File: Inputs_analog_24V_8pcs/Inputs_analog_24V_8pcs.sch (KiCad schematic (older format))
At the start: 14 parts, among them J1 Screw_Terminal_01x02, J2 Screw_Terminal_01x02, J3 Screw_Terminal_01x06, U1 SN74HC14N, U2 SN74HC14N, U3 74HC151N.652

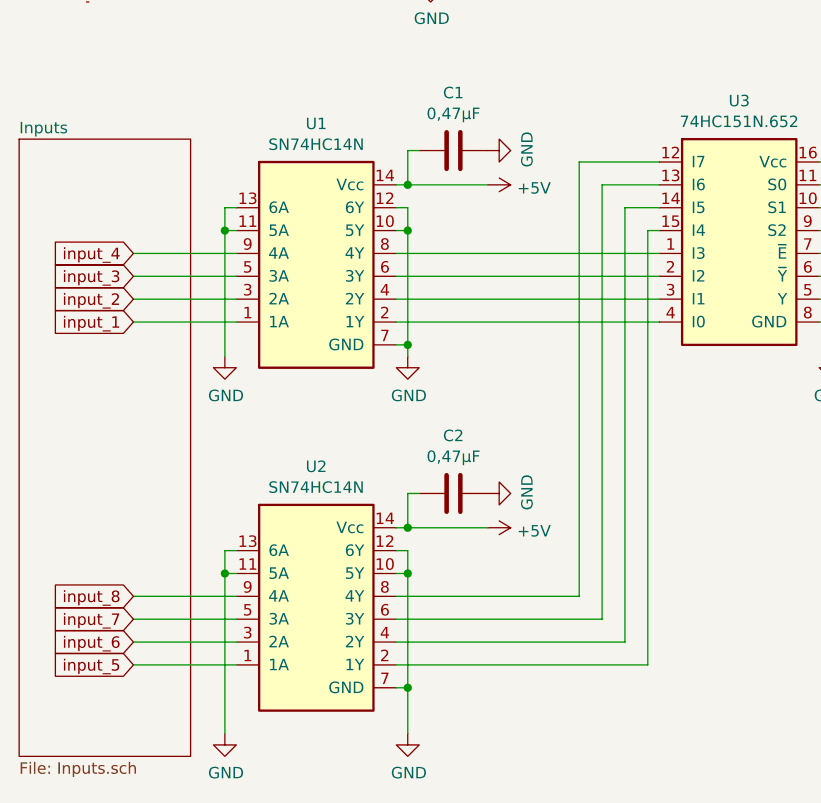
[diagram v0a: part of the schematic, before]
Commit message: Update pcb
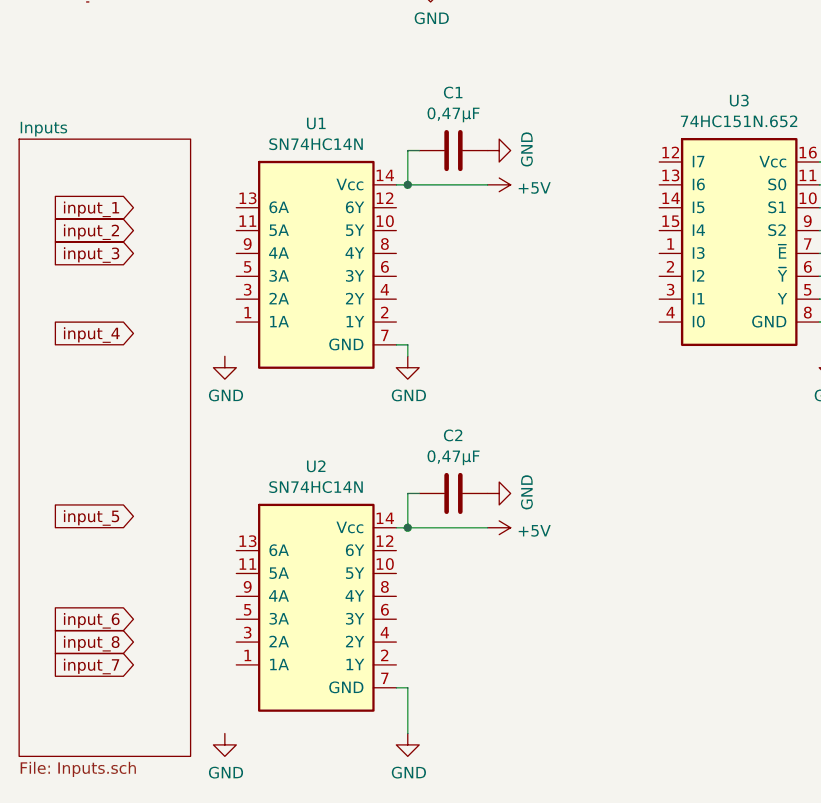
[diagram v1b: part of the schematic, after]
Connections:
- net GND: no longer U1.10 (5Y), U1.11 (5A), U1.12 (6Y), U1.13 (6A), U2.10 (5Y), U2.11 (5A), U2.12 (6Y), U2.13 (6A)
- net input_1: no longer U1.1 (1A)
- net input_2: no longer U1.3 (2A)
- net input_3: no longer U1.5 (3A)
- net input_4: no longer U1.9 (4A)
- net input_5: no longer U2.1 (1A)
- net input_6: no longer U2.3 (2A)
- net input_7: no longer U2.5 (3A)
- net input_8: no longer U2.9 (4A)
- net at U1.2 (1Y): no longer U3.4 (I0)
- net at U1.4 (2Y): no longer U3.3 (I1)
- net at U1.6 (3Y): no longer U3.2 (I2)
- net at U1.8 (4Y): no longer U3.1 (I3)
- net at U2.2 (1Y): no longer U3.15 (I4)
- net at U2.4 (2Y): no longer U3.14 (I5)
- net at U2.6 (3Y): no longer U3.13 (I6)
- net at U2.8 (4Y): no longer U3.12 (I7)
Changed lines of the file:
@@
 F1 "Inputs.sch" 50
 $EndSheet
-Text GLabel 1500 3900 0    50   Input ~ 0
+Text GLabel 1500 3400 0    50   Input ~ 0
 input_1
-Text GLabel 1500 3800 0    50   Input ~ 0
+Text GLabel 1500 3500 0    50   Input ~ 0
 input_2
-Text GLabel 1500 3700 0    50   Input ~ 0
+Text GLabel 1500 3600 0    50   Input ~ 0
 input_3
-Text GLabel 1500 3600 0    50   Input ~ 0
+Text GLabel 1500 3950 0    50   Input ~ 0
 input_4
+Text GLabel 1500 4750 0    50   Input ~ 0
+input_5
+Text GLabel 1500 5200 0    50   Input ~ 0
+input_6
 Text GLabel 1500 5400 0    50   Input ~ 0
-input_5
+input_7
 Text GLabel 1500 5300 0    50   Input ~ 0
-input_6
-Wire Wire Line
-	1500 3600 1950 3600
-Wire Wire Line
-	1500 3700 1950 3700
-Wire Wire Line
-	1500 3800 1950 3800
-Wire Wire Line
-	1500 3900 1950 3900
-Text GLabel 1500 5200 0    50   Input ~ 0
-input_7
-Text GLabel 1500 5100 0    50   Input ~ 0
 input_8
-Wire Wire Line
-	1500 5300 1950 5300
-Wire Wire Line
-	1500 5400 1950 5400
 $Comp
 L power:GND #PWR04
@@
 	1    0    0    -1
 $EndComp
-Wire Wire Line
-	1900 4900 1950 4900
-Wire Wire Line
-	1950 5000 1900 5000
-Connection ~ 1900 5000
-Wire Wire Line
-	1900 5000 1900 4900
 $Comp
 L power:+5V #PWR09
@@
 Wire Wire Line
 	2700 5500 2700 5700
-Connection ~ 2700 5500
-Wire Wire Line
-	2650 5000 2700 5000
-Wire Wire Line
-	2650 4900 2700 4900
-Wire Wire Line
-	2700 4900 2700 5000
-Connection ~ 2700 5000
 $Comp
 L power:+5V #PWR011
@@
 Wire Wire Line
 	4550 3900 4550 4050
-Wire Wire Line
-	1900 5000 1900 5700
-Wire Wire Line
-	1500 5200 1950 5200
-Wire Wire Line
-	1500 5100 1950 5100
 $Comp
 L power:GND #PWR03
@@
 $EndComp
 Wire Wire Line
-	1950 3500 1900 3500
-Wire Wire Line
-	1900 3500 1900 4050
-Wire Wire Line
-	1950 3400 1900 3400
-Wire Wire Line
-	1900 3400 1900 3500
-Connection ~ 1900 3500
-Wire Wire Line
-	2650 3500 2700 3500
-Wire Wire Line
-	2700 3500 2700 4000
-Connection ~ 2700 4000
-Wire Wire Line
-	2650 3400 2700 3400
-Wire Wire Line
-	2700 3400 2700 3500
-Connection ~ 2700 3500
-Wire Wire Line
-	3750 5400 3750 3500
-Wire Wire Line
-	3750 3500 3800 3500
-Wire Wire Line
-	3650 5300 3650 3400
-Wire Wire Line
-	3650 3400 3800 3400
-Wire Wire Line
-	3800 3300 3550 3300
-Wire Wire Line
-	3550 3300 3550 5200
-Wire Wire Line
-	3450 5100 3450 3200
-Wire Wire Line
-	3450 3200 3800 3200
-Wire Wire Line
-	2650 5100 3450 5100
-Wire Wire Line
-	2650 5200 3550 5200
-Wire Wire Line
-	2650 5300 3650 5300
-Wire Wire Line
-	2700 5000 2700 5500
-Wire Wire Line
-	3750 5400 2650 5400
-Wire Wire Line
-	2650 3600 3800 3600
-Wire Wire Line
-	2650 3700 3800 3700
-Wire Wire Line
-	2650 3800 3800 3800
-Wire Wire Line
-	2650 3900 3800 3900
-Wire Wire Line
 	4500 3300 4750 3300

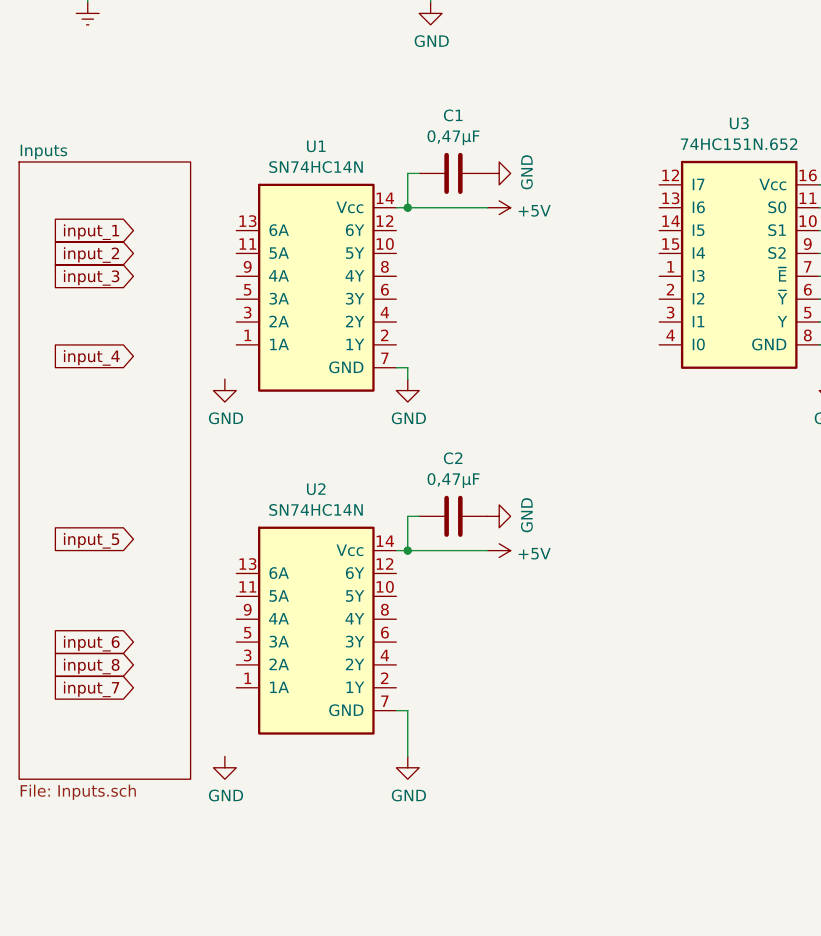
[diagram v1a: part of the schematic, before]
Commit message: Update pcb
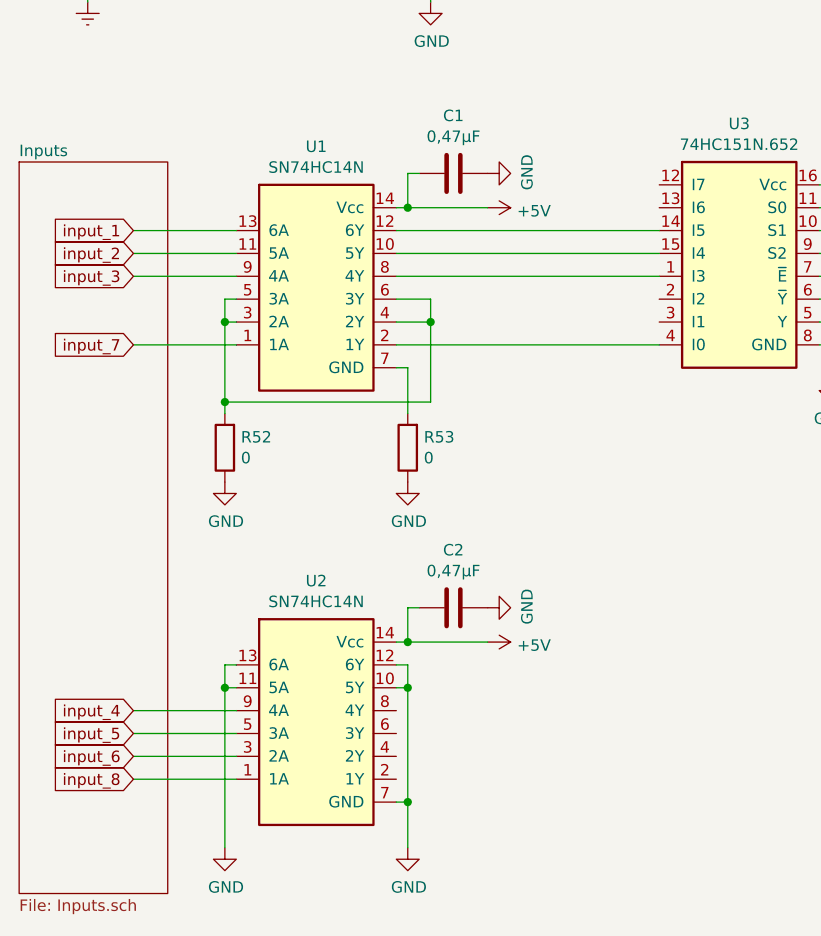
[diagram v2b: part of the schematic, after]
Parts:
- added R52, R53: 0, Resistor_THT:R_Axial_DIN0207_L6.3mm_D2.5mm_P7.62mm_Horizontal, symbol Device:R
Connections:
- net GND: now also U2.10 (5Y), U2.11 (5A), U2.12 (6Y), U2.13 (6A), R52.1, R53.1; no longer U1.7 (GND)
- net input_1: now also U1.13 (6A)
- net input_2: now also U1.11 (5A)
- net input_3: now also U1.9 (4A)
- net input_4: now also U2.9 (4A)
- net input_5: now also U2.5 (3A)
- net input_6: now also U2.3 (2A)
- net input_7: now also U1.1 (1A)
- net input_8: now also U2.1 (1A)
- net at U1.10 (5Y): now also U3.15 (I4)
- net at U1.12 (6Y): now also U3.14 (I5)
- net at U1.2 (1Y): now also U3.4 (I0)
- net at U1.3 (2A): now also U1.4 (2Y), U1.5 (3A), U1.6 (3Y), R52.2
- net at U1.8 (4Y): now also U3.1 (I3)
- new net: R53.2, U1.7 (GND)
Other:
- moved on the sheet: C2, U2
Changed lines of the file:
@@
 L Inputs_library:SN74HC14N U2
 U 1 1 5EA6DB6E
-P 2550 5950
-F 0 "U2" H 2300 7367 50  0000 C CNN
-F 1 "SN74HC14N" H 2300 7276 50  0000 C CNN
-F 2 "Package_DIP:DIP-14_W7.62mm" H 2550 5950 50  0001 C CNN
-F 3 "" H 2550 5950 50  0001 C CNN
-	1    2550 5950
+P 2550 6350
+F 0 "U2" H 2300 7767 50  0000 C CNN
+F 1 "SN74HC14N" H 2300 7676 50  0000 C CNN
+F 2 "Package_DIP:DIP-14_W7.62mm" H 2550 6350 50  0001 C CNN
+F 3 "" H 2550 6350 50  0001 C CNN
+	1    2550 6350
 	1    0    0    -1
 $EndComp
@@
 $EndComp
 $Sheet
-S 1000 3100 750  2700
+S 1000 3100 650  3200
 U 5EB670BF
 F0 "Inputs" 50
@@
 Text GLabel 1500 3600 0    50   Input ~ 0
 input_3
-Text GLabel 1500 3950 0    50   Input ~ 0
+Text GLabel 1500 5500 0    50   Input ~ 0
 input_4
-Text GLabel 1500 4750 0    50   Input ~ 0
+Text GLabel 1500 5600 0    50   Input ~ 0
 input_5
-Text GLabel 1500 5200 0    50   Input ~ 0
+Text GLabel 1500 5700 0    50   Input ~ 0
 input_6
-Text GLabel 1500 5400 0    50   Input ~ 0
+Text GLabel 1500 3900 0    50   Input ~ 0
 input_7
-Text GLabel 1500 5300 0    50   Input ~ 0
+Text GLabel 1500 5800 0    50   Input ~ 0
 input_8
 $Comp
 L power:GND #PWR04
 U 1 1 5EB7A823
-P 1900 5700
-F 0 "#PWR04" H 1900 5450 50  0001 C CNN
-F 1 "GND" H 1905 5527 50  0000 C CNN
-F 2 "" H 1900 5700 50  0001 C CNN
-F 3 "" H 1900 5700 50  0001 C CNN
-	1    1900 5700
+P 1900 6100
+F 0 "#PWR04" H 1900 5850 50  0001 C CNN
+F 1 "GND" H 1905 5927 50  0000 C CNN
+F 2 "" H 1900 6100 50  0001 C CNN
+F 3 "" H 1900 6100 50  0001 C CNN
+	1    1900 6100
 	1    0    0    -1
 $EndComp
@@
 L power:GND #PWR06
 U 1 1 5EBDD6D8
-P 2700 5700
-F 0 "#PWR06" H 2700 5450 50  0001 C CNN
-F 1 "GND" H 2705 5527 50  0000 C CNN
-F 2 "" H 2700 5700 50  0001 C CNN
-F 3 "" H 2700 5700 50  0001 C CNN
-	1    2700 5700
-	1    0    0    -1
-$EndComp
-Wire Wire Line
-	2650 5500 2700 5500
-Wire Wire Line
-	2700 5500 2700 5700
+P 2700 6100
+F 0 "#PWR06" H 2700 5850 50  0001 C CNN
+F 1 "GND" H 2705 5927 50  0000 C CNN
+F 2 "" H 2700 6100 50  0001 C CNN
+F 3 "" H 2700 6100 50  0001 C CNN
+	1    2700 6100
+	1    0    0    -1
+$EndComp
+Wire Wire Line
+	2650 5900 2700 5900
+Wire Wire Line
+	2700 5900 2700 6100
 $Comp
 L power:+5V #PWR011
 U 1 1 5EBE4E40
-P 3050 4800
-F 0 "#PWR011" H 3050 4650 50  0001 C CNN
-F 1 "+5V" V 3065 4928 50  0000 L CNN
-F 2 "" H 3050 4800 50  0001 C CNN
-F 3 "" H 3050 4800 50  0001 C CNN
-	1    3050 4800
-	0    1    1    0
-$EndComp
-Wire Wire Line
-	2650 4800 2700 4800
+P 3050 5200
+F 0 "#PWR011" H 3050 5050 50  0001 C CNN
+F 1 "+5V" V 3065 5328 50  0000 L CNN
+F 2 "" H 3050 5200 50  0001 C CNN
+F 3 "" H 3050 5200 50  0001 C CNN
+	1    3050 5200
+	0    1    1    0
+$EndComp
+Wire Wire Line
+	2650 5200 2700 5200
 $Comp
 L Device:C C2
 U 1 1 5EBE4E47
-P 2900 4650
-F 0 "C2" V 2648 4650 50  0000 C CNN
-F 1 "0,47μF" V 2739 4650 50  0000 C CNN
-F 2 "Capacitor_THT:C_Disc_D4.3mm_W1.9mm_P5.00mm" H 2938 4500 50  0001 C CNN
-F 3 "~" H 2900 4650 50  0001 C CNN
-	1    2900 4650
-	0    1    1    0
-$EndComp
-Wire Wire Line
-	2750 4650 2700 4650
-Wire Wire Line
-	2700 4650 2700 4800
-Connection ~ 2700 4800
+P 2900 5050
+F 0 "C2" V 2648 5050 50  0000 C CNN
+F 1 "0,47μF" V 2739 5050 50  0000 C CNN
+F 2 "Capacitor_THT:C_Disc_D4.3mm_W1.9mm_P5.00mm" H 2938 4900 50  0001 C CNN
+F 3 "~" H 2900 5050 50  0001 C CNN
+	1    2900 5050
+	0    1    1    0
+$EndComp
+Wire Wire Line
+	2750 5050 2700 5050
+Wire Wire Line
+	2700 5050 2700 5200
+Connection ~ 2700 5200
 $Comp
 L power:GND #PWR010
 U 1 1 5EBE4E50
-P 3050 4650
-F 0 "#PWR010" H 3050 4400 50  0001 C CNN
-F 1 "GND" H 3055 4477 50  0000 C CNN
-F 2 "" H 3050 4650 50  0001 C CNN
-F 3 "" H 3050 4650 50  0001 C CNN
-	1    3050 4650
+P 3050 5050
+F 0 "#PWR010" H 3050 4800 50  0001 C CNN
+F 1 "GND" H 3055 4877 50  0000 C CNN
+F 2 "" H 3050 5050 50  0001 C CNN
+F 3 "" H 3050 5050 50  0001 C CNN
+	1    3050 5050
 	0    -1   -1   0
 $EndComp
 Wire Wire Line
-	2700 4800 3050 4800
-$Comp
-L power:GND #PWR05
-U 1 1 5EBE68A6
-P 2700 4050
-F 0 "#PWR05" H 2700 3800 50  0001 C CNN
-F 1 "GND" H 2705 3877 50  0000 C CNN
-F 2 "" H 2700 4050 50  0001 C CNN
-F 3 "" H 2700 4050 50  0001 C CNN
-	1    2700 4050
-	1    0    0    -1
-$EndComp
-Wire Wire Line
-	2650 4000 2700 4000
-Wire Wire Line
-	2700 4000 2700 4050
+	2700 5200 3050 5200
 $Comp
 L power:+5V #PWR015
@@
 L power:GND #PWR03
 U 1 1 5EC164A3
-P 1900 4050
-F 0 "#PWR03" H 1900 3800 50  0001 C CNN
-F 1 "GND" H 1905 3877 50  0000 C CNN
-F 2 "" H 1900 4050 50  0001 C CNN
-F 3 "" H 1900 4050 50  0001 C CNN
-	1    1900 4050
+P 1900 4500
+F 0 "#PWR03" H 1900 4250 50  0001 C CNN
+F 1 "GND" H 1905 4327 50  0000 C CNN
+F 2 "" H 1900 4500 50  0001 C CNN
+F 3 "" H 1900 4500 50  0001 C CNN
+	1    1900 4500
 	1    0    0    -1
 $EndComp
@@
 	1    0    0    -1
 $EndComp
+Wire Wire Line
+	1500 3400 1950 3400
+Wire Wire Line
+	1500 3500 1950 3500
+Wire Wire Line
+	1500 3600 1950 3600
+Wire Wire Line
+	2650 3400 3800 3400
+Wire Wire Line
+	2650 3500 3800 3500
+Wire Wire Line
+	2650 3600 3800 3600
+Wire Wire Line
+	1500 3900 1950 3900
+Wire Wire Line
+	2650 3900 3800 3900
+$Comp
+L power:GND #PWR07
+U 1 1 5E7B992E
+P 2700 4500
+F 0 "#PWR07" H 2700 4250 50  0001 C CNN
+F 1 "GND" H 2705 4327 50  0000 C CNN
+F 2 "" H 2700 4500 50  0001 C CNN
+F 3 "" H 2700 4500 50  0001 C CNN
+	1    2700 4500
+	1    0    0    -1
+$EndComp
+$Comp
+L Device:R R52
+U 1 1 5E81BB40
+P 1900 4350
+F 0 "R52" H 1830 4304 50  0000 R CNN
+F 1 "0" H 1830 4395 50  0000 R CNN
+F 2 "Resistor_THT:R_Axial_DIN0207_L6.3mm_D2.5mm_P7.62mm_Horizontal" V 1830 4350 50  0001 C CNN
+F 3 "~" H 1900 4350 50  0001 C CNN
+	1    1900 4350
+	-1   0    0    1
+$EndComp
+$Comp
+L Device:R R53
+U 1 1 5E841327
+P 2700 4350
+F 0 "R53" H 2630 4304 50  0000 R CNN
+F 1 "0" H 2630 4395 50  0000 R CNN
+F 2 "Resistor_THT:R_Axial_DIN0207_L6.3mm_D2.5mm_P7.62mm_Horizontal" V 2630 4350 50  0001 C CNN
+F 3 "~" H 2700 4350 50  0001 C CNN
+	1    2700 4350
+	-1   0    0    1
+$EndComp
+Wire Wire Line
+	2650 4000 2700 4000
+Wire Wire Line
+	2700 4000 2700 4200
+Wire Wire Line
+	2650 3700 2800 3700
+Wire Wire Line
+	2800 3700 2800 3800
+Wire Wire Line
+	2800 4150 1900 4150
+Wire Wire Line
+	1900 4150 1900 4200
+Wire Wire Line
+	2650 3800 2800 3800
+Connection ~ 2800 3800
+Wire Wire Line
+	2800 3800 2800 4150
+Wire Wire Line
+	1950 3700 1900 3700
+Wire Wire Line
+	1900 3700 1900 3800
+Connection ~ 1900 4150
+Wire Wire Line
+	1950 3800 1900 3800
+Connection ~ 1900 3800
+Wire Wire Line
+	1900 3800 1900 4150
+Wire Wire Line
+	1500 5500 1950 5500
+Wire Wire Line
+	2650 5300 2700 5300
+Wire Wire Line
+	2700 5300 2700 5400
+Wire Wire Line
+	2700 5400 2650 5400
+Wire Wire Line
+	1950 5300 1900 5300
+Wire Wire Line
+	1900 5300 1900 5400
+Wire Wire Line
+	1900 5400 1950 5400
+Wire Wire Line
+	2700 5400 2700 5900
+Connection ~ 2700 5400
+Connection ~ 2700 5900
+Wire Wire Line
+	1900 5400 1900 6100
+Connection ~ 1900 5400
+Wire Wire Line
+	1500 5800 1950 5800
+Wire Wire Line
+	1500 5700 1950 5700
+Wire Wire Line
+	1500 5600 1950 5600
 $EndSCHEMATC
